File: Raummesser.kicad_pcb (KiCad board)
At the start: 2 copper layers, 57 x 52 mm, 12 parts, among them J1 USB_C_Receptacle_USB2.0_16P, J2 Display, U1 ESP32-C3-WROOM-02, U2 SCD40-D-R2, U3 AP2112K-3.3

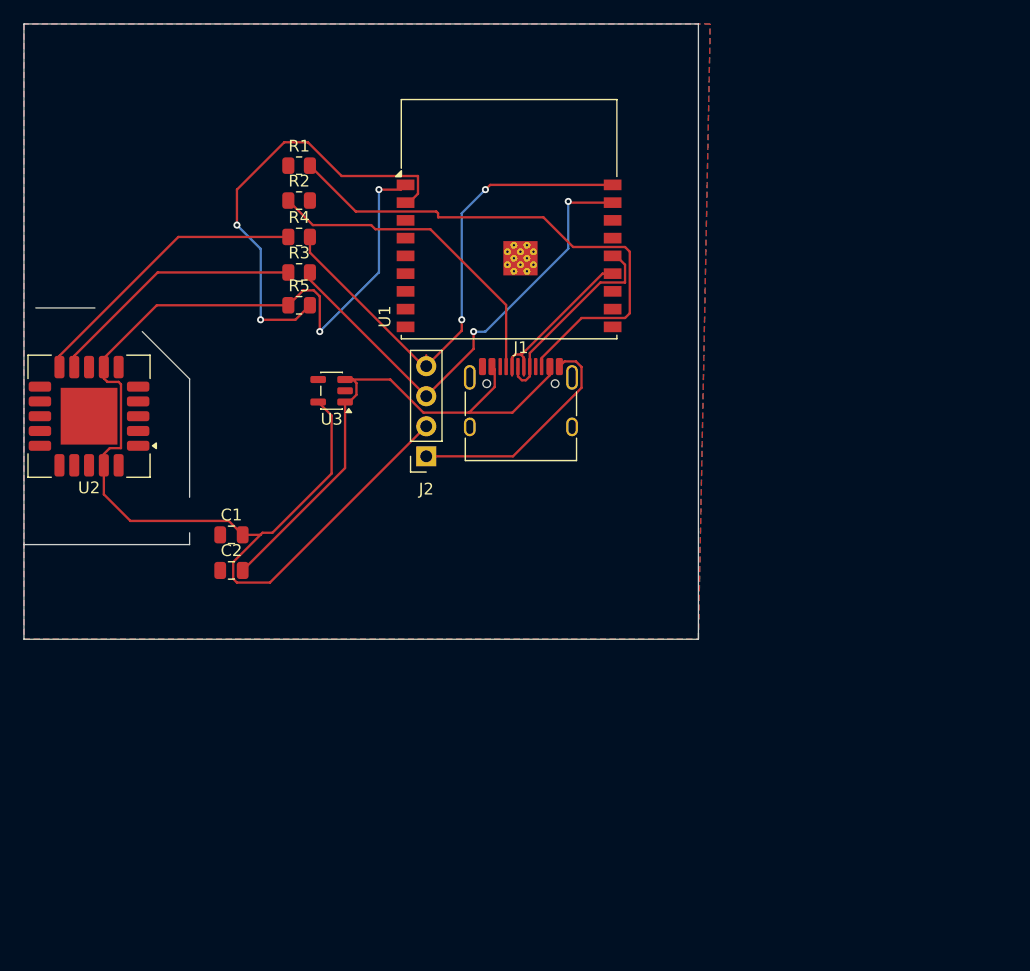
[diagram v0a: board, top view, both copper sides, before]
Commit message: Add files via upload
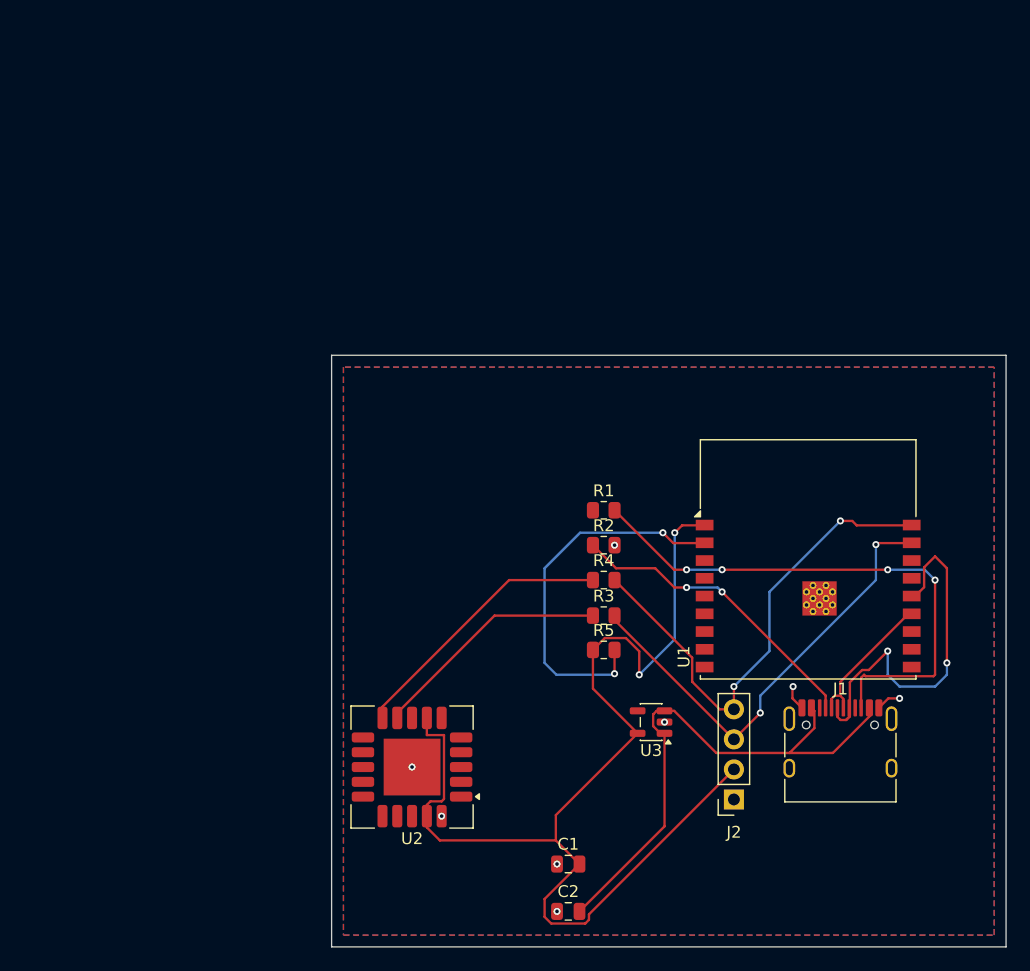
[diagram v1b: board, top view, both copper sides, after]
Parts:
- moved C2 40.5 mm to (172.0, 144.0)
- moved U2 40.3 mm to (158.8, 131.8)
- moved C1 39.8 mm to (172.0, 140.0)
- moved J1 39.5 mm to (195.0, 130.8)
- moved J2 38.9 mm to (186.0, 134.5)
- moved U3 38.9 mm to (179.0, 128.0)
- moved R1 38.9 mm to (175.0, 110.1)
- moved R2 38.9 mm to (175.0, 113.0)
- moved R5 38.9 mm to (175.0, 121.9)
- moved R3 38.8 mm to (175.0, 119.0)
- moved R4 38.8 mm to (175.0, 116.0)
- moved U1 38.3 mm to (192.3, 117.3)
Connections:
- J1 pad A6: Net-(U1-IO19) -> Net-(J1-CC1)
- J1 pad B6: Net-(U1-IO19) -> Net-(J1-CC1)
- U1 pad 14: Net-(U1-IO19) -> Net-(J1-CC1)
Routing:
- net Net-(J1-CC1): track 27.3 -> 59.2 mm, vias 0 -> 4
- net Net-(U1-IO19): track 17.4 -> 0.00 mm
- net GND: track 19.5 -> 4.23 mm, vias 0 -> 8
- net Net-(J2-Pin_2): track 110.5 -> 96.9 mm
- net Net-(U1-EN): track 37.5 -> 31.5 mm
- net Net-(U1-IO18): track 14.8 -> 12.3 mm
- net Net-(J2-Pin_4): track 44.0 -> 41.6 mm
- net Net-(U2-SCL): track 22.0 -> 20.4 mm
- net Net-(J2-Pin_3): track 40.5 -> 39.1 mm
- net Net-(J1-CC2): track 45.2 -> 46.5 mm, vias 0 -> 4
- net Net-(U2-SDA): track 24.5 -> 23.2 mm
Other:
- board size 57 x 52 mm -> 57 x 50 mm
